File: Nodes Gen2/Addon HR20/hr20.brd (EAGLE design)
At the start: 70 x 48 mm, 12 parts, among them SW1 430186043916, SW2 430186043916, SW3 430186043916

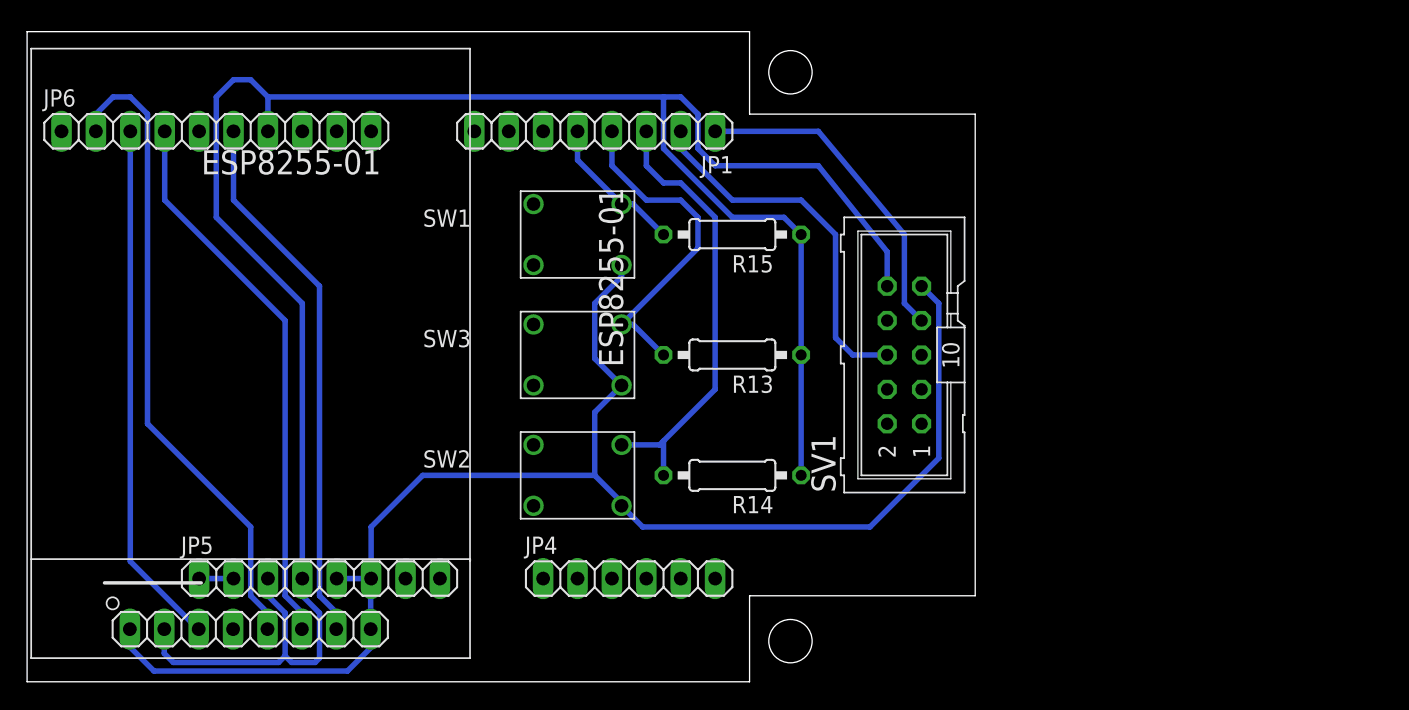
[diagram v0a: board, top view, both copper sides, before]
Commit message: gen 2 dev + bom
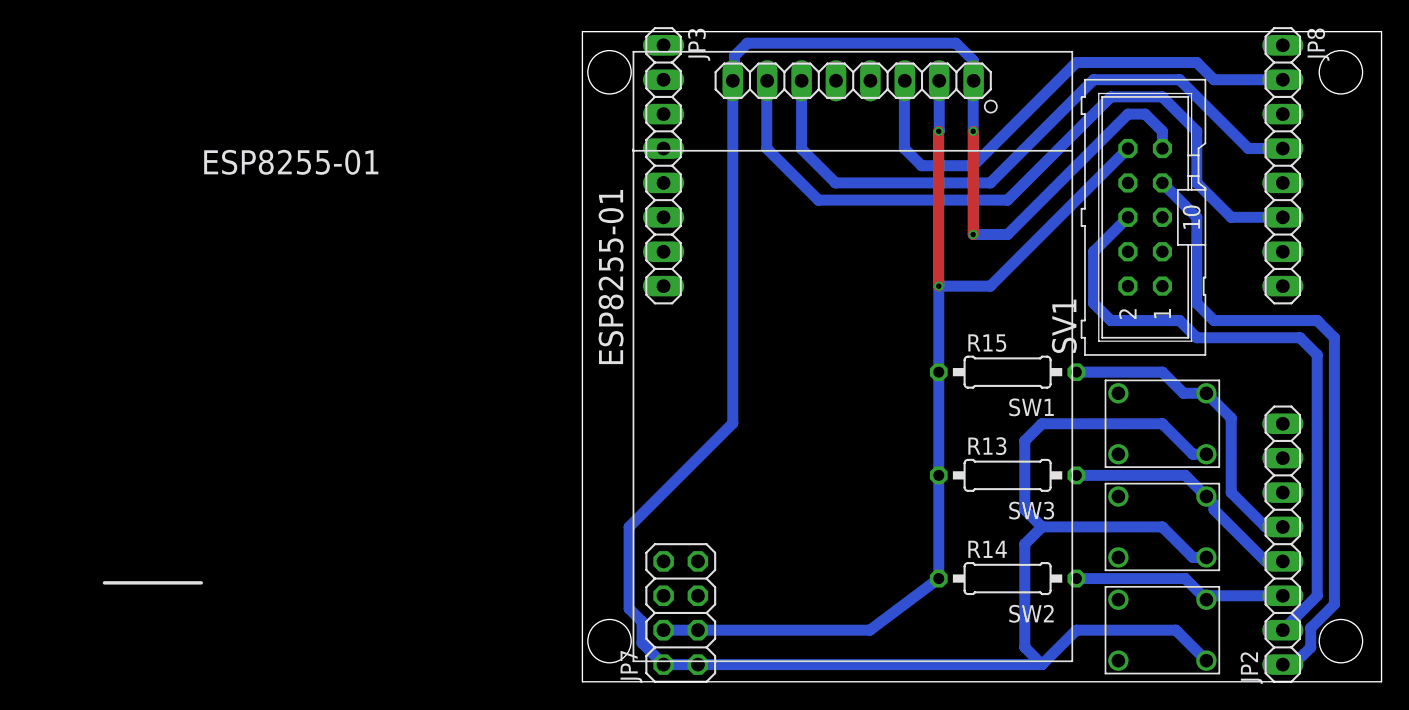
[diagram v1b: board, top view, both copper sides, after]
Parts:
- removed JP1, JP5: (no value), pinhead:1X08
- removed JP4: (no value), pinhead:1X06
- removed JP6: (no value), pinhead:1X10
- added JP2, JP3, JP8: (no value), pinhead:1X08
- added JP7: (no value), pinhead:2X04
- moved U$2 88.9 mm to (77.2, 46.5), turned to 180 degrees
- moved SW1 45.4 mm to (83.8, 19.1)
- moved SW3 45.0 mm to (83.8, 11.4)
- moved SW2 44.7 mm to (83.8, 3.81)
- moved R15 22.7 mm to (72.4, 22.9), turned to 0 degrees
- moved R13 22.2 mm to (72.4, 15.2), turned to 0 degrees
- moved R14 21.7 mm to (72.4, 7.62), turned to 0 degrees
- moved SV1 20.5 mm to (82.5, 34.3)
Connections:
- removed net A4_SDA1: JP6.9
- removed net A4_SDA2: JP4.5
- removed net A5_SCL1: JP6.10
- removed net A5_SCL2: JP4.6
- removed net A6: JP5.8
- removed net A7: JP5.7
- removed net AREF: JP6.8
- removed net D8: JP6.1
- removed net D9: JP6.2, U$2.5
- new net A4_SDA: JP3.5
- new net A5_SCL: JP3.6
- new net D8_SS: JP8.1, U$2.3
- new net D9_SS: JP8.2
- new net RESERVE2: JP8.8
- net A0: now also JP3.1; no longer JP4.1
- net A1: now also JP3.2; no longer JP4.2
- net A2: now also JP3.3; no longer JP4.3
- net A3_V24: now also JP3.4; no longer JP4.4
- net D10_SS: now also JP8.3; no longer JP6.3, U$2.3
- net D11_MOSI: now also JP8.4; no longer JP6.4
- net D12_MISO: now also JP8.5; no longer JP6.5
- net D13_SCK: now also JP8.6; no longer JP6.6
- net D2: now also JP2.3; no longer JP1.3
- net D3: now also JP2.4; no longer JP1.4
- net D4: now also JP2.5; no longer JP1.5
- net D5: now also JP2.6; no longer JP1.6
- net D6: now also JP2.7; no longer JP1.7
- net D7: now also JP2.8; no longer JP1.8
- net GND: now also JP7.3, JP7.4; no longer JP5.3, JP5.4, JP6.7
- net P24P: now also JP7.7, JP7.8; no longer JP5.1, JP5.2
- net P5V: now also JP7.1, JP7.2; no longer JP5.5, JP5.6
- net RESET: now also JP8.7
- net RX: now also JP2.1; no longer JP1.1
- net TX: now also JP2.2; no longer JP1.2
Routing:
- net GND: track 161.6 -> 76.5 mm, vias 0 -> 2
- net P5V: track 110.6 -> 188.2 mm, vias 0 -> 2
- net D9: track 47.9 -> 0.00 mm
- net D10_SS: track 38.9 -> 0.00 mm
- net D9_SS: track 0.00 -> 37.1 mm
- net RX: track 24.4 -> 47.3 mm
- net TX: track 27.3 -> 46.9 mm
- net D2: track 33.0 -> 16.0 mm
- net D13_SCK: track 39.9 -> 53.8 mm
- net D4: track 10.7 -> 23.2 mm
- net D3: track 24.7 -> 18.1 mm
- net D11_MOSI: track 41.0 -> 46.9 mm
- net P24P: track 2.54 -> 0.00 mm
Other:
- board size 70 x 48 mm -> 59 x 48 mm
